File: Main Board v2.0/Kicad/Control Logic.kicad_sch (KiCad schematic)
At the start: 24 parts, among them J2 +3V3 Supply, J3 JTAG, U7 XC95288XL-TQ144, U8 AP1117-33

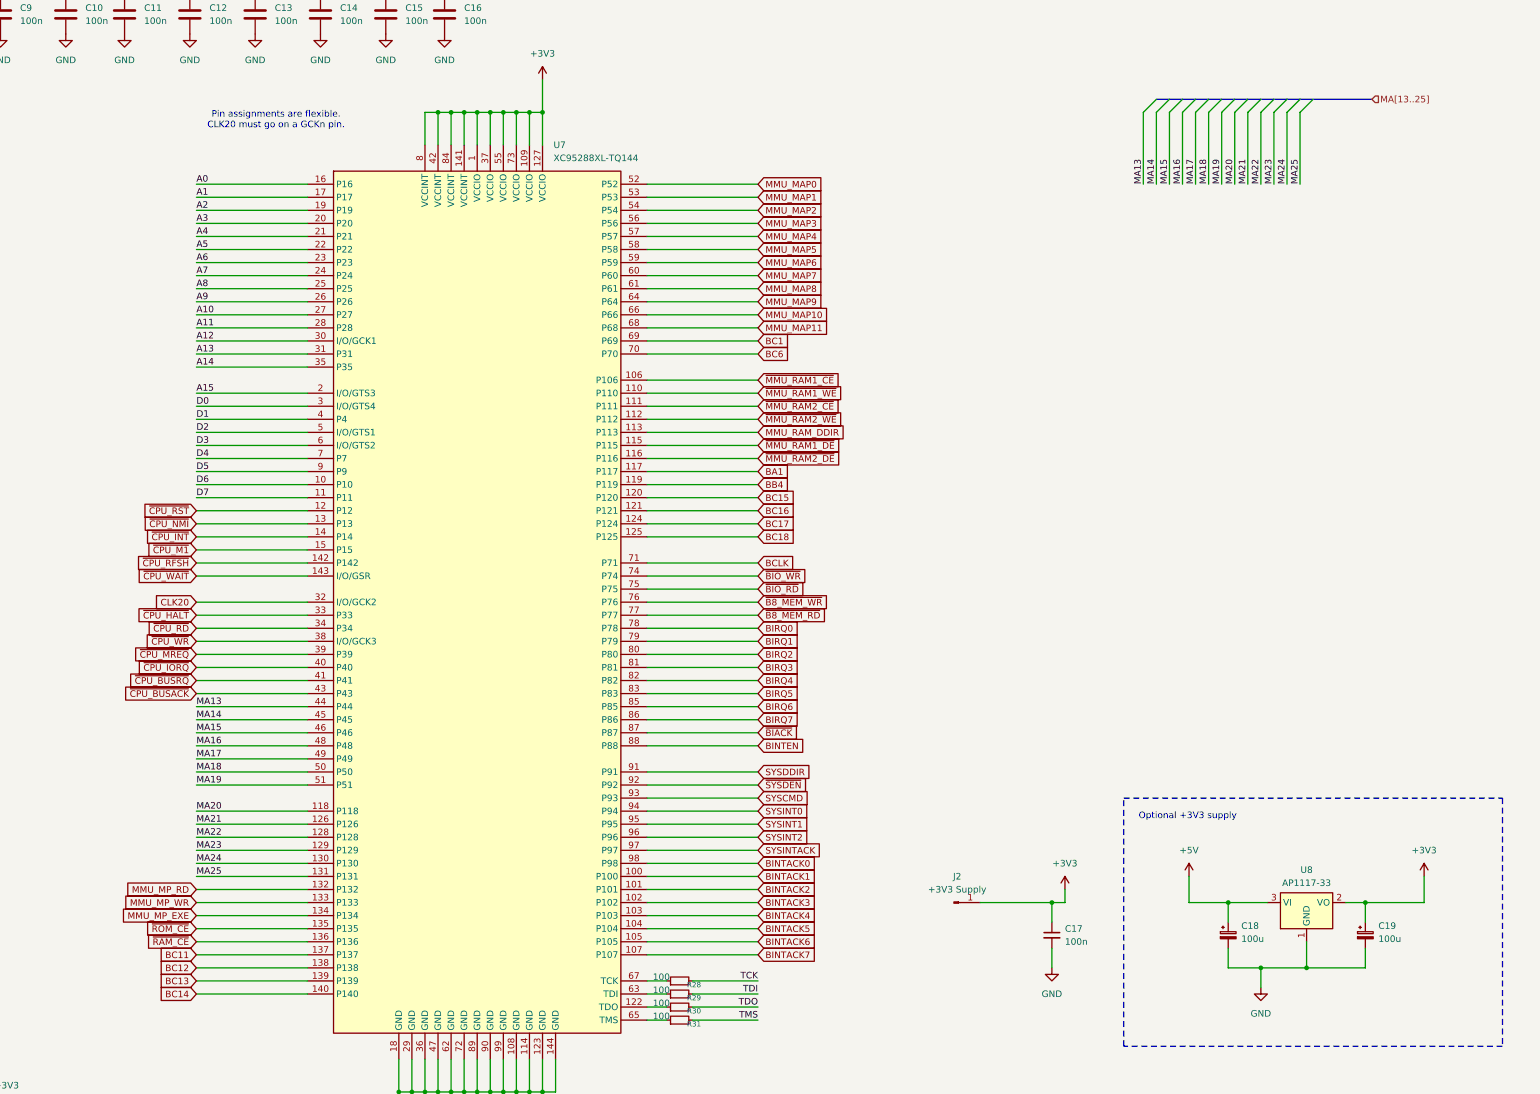
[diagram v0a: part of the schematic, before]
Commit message: board update
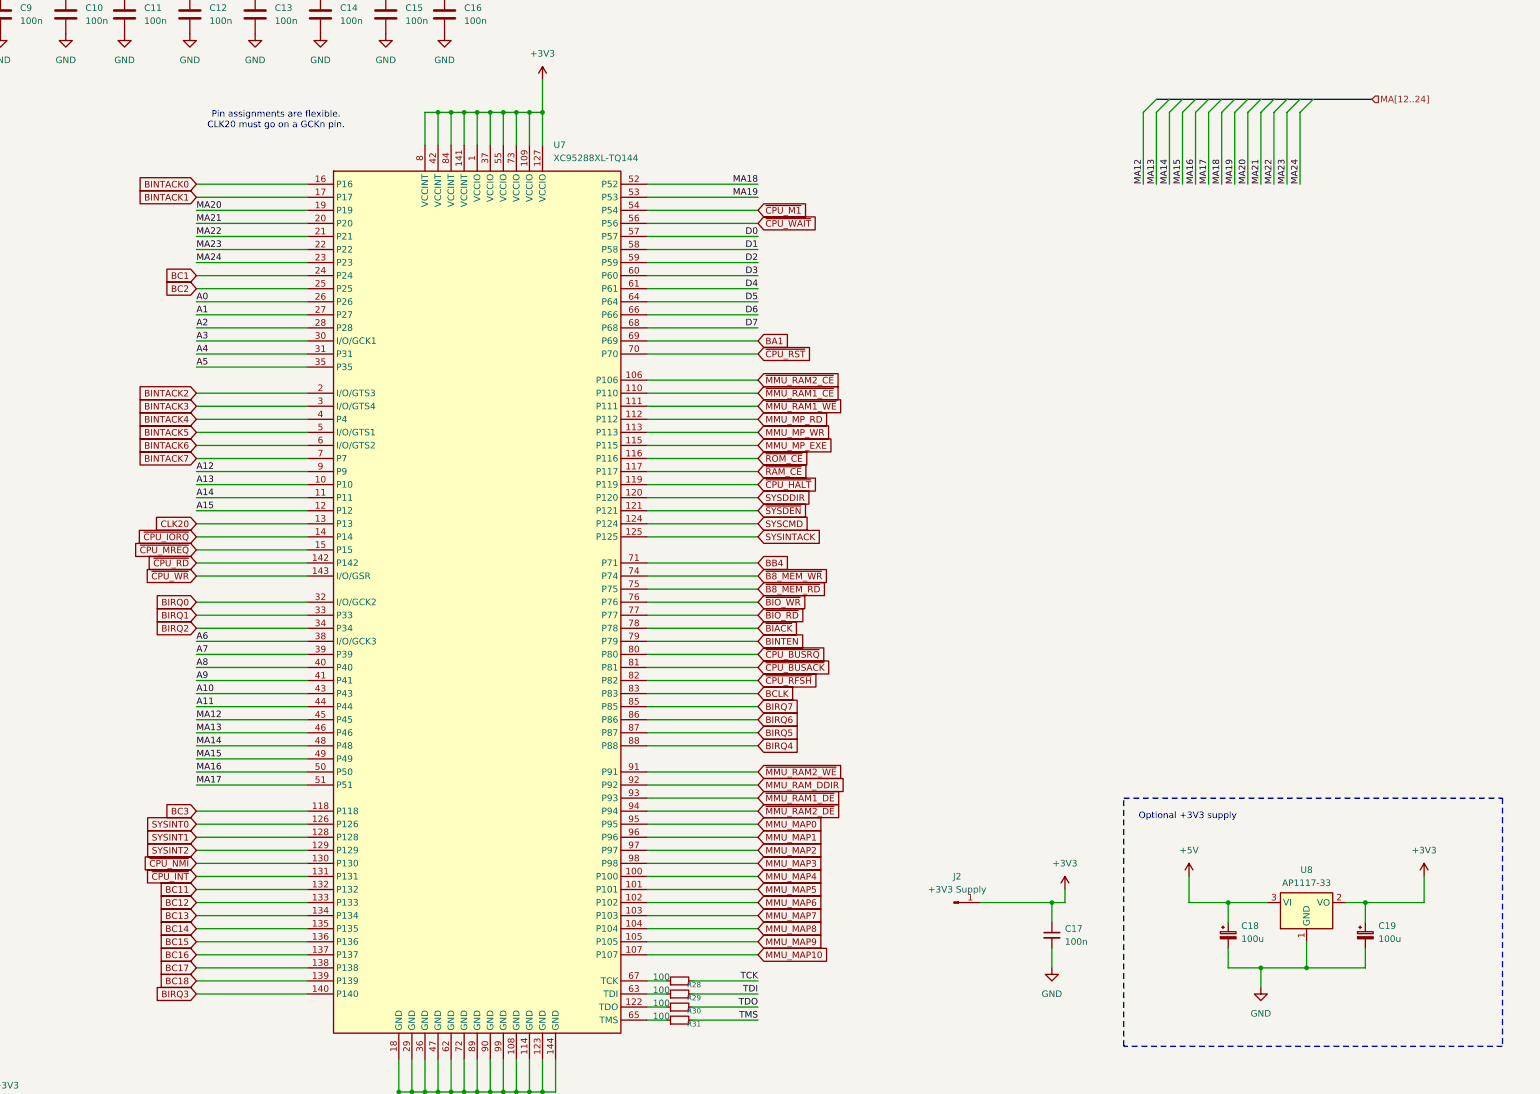
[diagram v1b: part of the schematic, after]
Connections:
- net BC6 is gone; now on net ~{CPU_RST}: U7.70 (P70)
- net MA25 is gone; now on net ~{CPU_INT}: U7.131 (P131)
- net MMU_MAP11 is gone; now on net D7: U7.68 (P68)
- net A0: now also U7.26 (P26); no longer U7.16 (P16)
- net A1: now also U7.27 (P27); no longer U7.17 (P17)
- net A10: now also U7.43 (P43); no longer U7.27 (P27)
- net A11: now also U7.44 (P44); no longer U7.28 (P28)
- net A12: now also U7.9 (P9); no longer U7.30 (I/O/GCK1)
- net A13: now also U7.10 (P10); no longer U7.31 (P31)
- net A14: now also U7.11 (P11); no longer U7.35 (P35)
- net A15: now also U7.12 (P12); no longer U7.2 (I/O/GTS3)
- net A2: now also U7.28 (P28); no longer U7.19 (P19)
- net A3: now also U7.30 (I/O/GCK1); no longer U7.20 (P20)
- net A4: now also U7.31 (P31); no longer U7.21 (P21)
- net A5: now also U7.35 (P35); no longer U7.22 (P22)
- net A6: now also U7.38 (I/O/GCK3); no longer U7.23 (P23)
- net A7: now also U7.39 (P39); no longer U7.24 (P24)
- net A8: now also U7.40 (P40); no longer U7.25 (P25)
- net A9: now also U7.41 (P41); no longer U7.26 (P26)
- net BA1: now also U7.69 (P69); no longer U7.117 (P117)
- net BB4: now also U7.71 (P71); no longer U7.119 (P119)
- net BC1: now also U7.24 (P24); no longer U7.69 (P69)
- net BC11: now also U7.132 (P132); no longer U7.137 (P137)
- net BC12: now also U7.133 (P133); no longer U7.138 (P138)
- net BC13: now also U7.134 (P134); no longer U7.139 (P139)
- net BC14: now also U7.135 (P135); no longer U7.140 (P140)
- net BC15: now also U7.136 (P136); no longer U7.120 (P120)
- net BC16: now also U7.137 (P137); no longer U7.121 (P121)
- net BC17: now also U7.138 (P138); no longer U7.124 (P124)
- net BC18: now also U7.139 (P139); no longer U7.125 (P125)
- net BCLK: now also U7.83 (P83); no longer U7.71 (P71)
- net BINTACK0: now also U7.16 (P16); no longer U7.98 (P98)
- net BINTACK1: now also U7.17 (P17); no longer U7.100 (P100)
- net BINTACK2: now also U7.2 (I/O/GTS3); no longer U7.101 (P101)
- net BINTACK3: now also U7.3 (I/O/GTS4); no longer U7.102 (P102)
- net BINTACK4: now also U7.4 (P4); no longer U7.103 (P103)
- net BINTACK5: now also U7.5 (I/O/GTS1); no longer U7.104 (P104)
- net BINTACK6: now also U7.6 (I/O/GTS2); no longer U7.105 (P105)
- net BINTACK7: now also U7.7 (P7); no longer U7.107 (P107)
- net BINTEN: now also U7.79 (P79); no longer U7.88 (P88)
- net BIRQ0: now also U7.32 (I/O/GCK2); no longer U7.78 (P78)
- net BIRQ1: now also U7.33 (P33); no longer U7.79 (P79)
- net BIRQ2: now also U7.34 (P34); no longer U7.80 (P80)
- net BIRQ3: now also U7.140 (P140); no longer U7.81 (P81)
- net BIRQ4: now also U7.88 (P88); no longer U7.82 (P82)
- net BIRQ5: now also U7.87 (P87); no longer U7.83 (P83)
- net BIRQ6: now also U7.86 (P86); no longer U7.85 (P85)
- net BIRQ7: now also U7.85 (P85); no longer U7.86 (P86)
- net CLK20: now also U7.13 (P13); no longer U7.32 (I/O/GCK2)
- net D0: now also U7.57 (P57); no longer U7.3 (I/O/GTS4)
- net D1: now also U7.58 (P58); no longer U7.4 (P4)
- net D2: now also U7.59 (P59); no longer U7.5 (I/O/GTS1)
- net D3: now also U7.60 (P60); no longer U7.6 (I/O/GTS2)
- net D4: now also U7.61 (P61); no longer U7.7 (P7)
- net D5: now also U7.64 (P64); no longer U7.9 (P9)
- net D6: now also U7.66 (P66); no longer U7.10 (P10)
- net D7: no longer U7.11 (P11)
- net MA13: now also U7.46 (P46); no longer U7.44 (P44)
- net MA14: now also U7.48 (P48); no longer U7.45 (P45)
- net MA15: now also U7.49 (P49); no longer U7.46 (P46)
- net MA16: now also U7.50 (P50); no longer U7.48 (P48)
- net MA17: now also U7.51 (P51); no longer U7.49 (P49)
- net MA18: now also U7.52 (P52); no longer U7.50 (P50)
- net MA19: now also U7.53 (P53); no longer U7.51 (P51)
- net MA20: now also U7.19 (P19); no longer U7.118 (P118)
- net MA21: now also U7.20 (P20); no longer U7.126 (P126)
- net MA22: now also U7.21 (P21); no longer U7.128 (P128)
- net MA23: now also U7.22 (P22); no longer U7.129 (P129)
- net MA24: now also U7.23 (P23); no longer U7.130 (P130)
- net MMU_MAP0: now also U7.95 (P95); no longer U7.52 (P52)
- net MMU_MAP1: now also U7.96 (P96); no longer U7.53 (P53)
- net MMU_MAP10: now also U7.107 (P107); no longer U7.66 (P66)
- net MMU_MAP2: now also U7.97 (P97); no longer U7.54 (P54)
- net MMU_MAP3: now also U7.98 (P98); no longer U7.56 (P56)
- net MMU_MAP4: now also U7.100 (P100); no longer U7.57 (P57)
- net MMU_MAP5: now also U7.101 (P101); no longer U7.58 (P58)
- net MMU_MAP6: now also U7.102 (P102); no longer U7.59 (P59)
- net MMU_MAP7: now also U7.103 (P103); no longer U7.60 (P60)
- net MMU_MAP8: now also U7.104 (P104); no longer U7.61 (P61)
- net MMU_MAP9: now also U7.105 (P105); no longer U7.64 (P64)
- net MMU_MP_EXE: now also U7.115 (P115); no longer U7.134 (P134)
- net MMU_MP_RD: now also U7.112 (P112); no longer U7.132 (P132)
- net MMU_MP_WR: now also U7.113 (P113); no longer U7.133 (P133)
- net MMU_RAM_DDIR: now also U7.92 (P92); no longer U7.113 (P113)
- net SYSCMD: now also U7.124 (P124); no longer U7.93 (P93)
- net SYSDDIR: now also U7.120 (P120); no longer U7.91 (P91)
- net SYSINT0: now also U7.126 (P126); no longer U7.94 (P94)
- net SYSINT1: now also U7.128 (P128); no longer U7.95 (P95)
- net SYSINT2: now also U7.129 (P129); no longer U7.96 (P96)
- net SYSINTACK: now also U7.125 (P125); no longer U7.97 (P97)
- net ~{B8_MEM_RD}: now also U7.75 (P75); no longer U7.77 (P77)
- net ~{B8_MEM_WR}: now also U7.74 (P74); no longer U7.76 (P76)
- net ~{BIACK}: now also U7.78 (P78); no longer U7.87 (P87)
- net ~{BIO_RD}: now also U7.77 (P77); no longer U7.75 (P75)
- net ~{BIO_WR}: now also U7.76 (P76); no longer U7.74 (P74)
- net ~{CPU_BUSACK}: now also U7.81 (P81); no longer U7.43 (P43)
- net ~{CPU_BUSRQ}: now also U7.80 (P80); no longer U7.41 (P41)
- net ~{CPU_HALT}: now also U7.119 (P119); no longer U7.33 (P33)
- net ~{CPU_INT}: no longer U7.14 (P14)
- net ~{CPU_IORQ}: now also U7.14 (P14); no longer U7.40 (P40)
- net ~{CPU_M1}: now also U7.54 (P54); no longer U7.15 (P15)
- net ~{CPU_MREQ}: now also U7.15 (P15); no longer U7.39 (P39)
- net ~{CPU_NMI}: now also U7.130 (P130); no longer U7.13 (P13)
- net ~{CPU_RD}: now also U7.142 (P142); no longer U7.34 (P34)
- net ~{CPU_RFSH}: now also U7.82 (P82); no longer U7.142 (P142)
- net ~{CPU_RST}: no longer U7.12 (P12)
- net ~{CPU_WAIT}: now also U7.56 (P56); no longer U7.143 (I/O/GSR)
- net ~{CPU_WR}: now also U7.143 (I/O/GSR); no longer U7.38 (I/O/GCK3)
- net ~{MMU_RAM1_CE}: now also U7.110 (P110); no longer U7.106 (P106)
- net ~{MMU_RAM1_DE}: now also U7.93 (P93); no longer U7.115 (P115)
- net ~{MMU_RAM1_WE}: now also U7.111 (P111); no longer U7.110 (P110)
- net ~{MMU_RAM2_CE}: now also U7.106 (P106); no longer U7.111 (P111)
- net ~{MMU_RAM2_DE}: now also U7.94 (P94); no longer U7.116 (P116)
- net ~{MMU_RAM2_WE}: now also U7.91 (P91); no longer U7.112 (P112)
- net ~{RAM_CE}: now also U7.117 (P117); no longer U7.136 (P136)
- net ~{ROM_CE}: now also U7.116 (P116); no longer U7.135 (P135)
- net ~{SYSDEN}: now also U7.121 (P121); no longer U7.92 (P92)
- new net BC2: U7.25 (P25)
- new net BC3: U7.118 (P118)
- new net MA12: U7.45 (P45)
